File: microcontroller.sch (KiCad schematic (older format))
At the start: 25 parts, among them Q1 DMN62D0U-7, U5 MCP2221A, U6 ESP32, U7 NPIC6C596ADJ, U8 NPIC6C596ADJ, U9 NPIC6C596ADJ

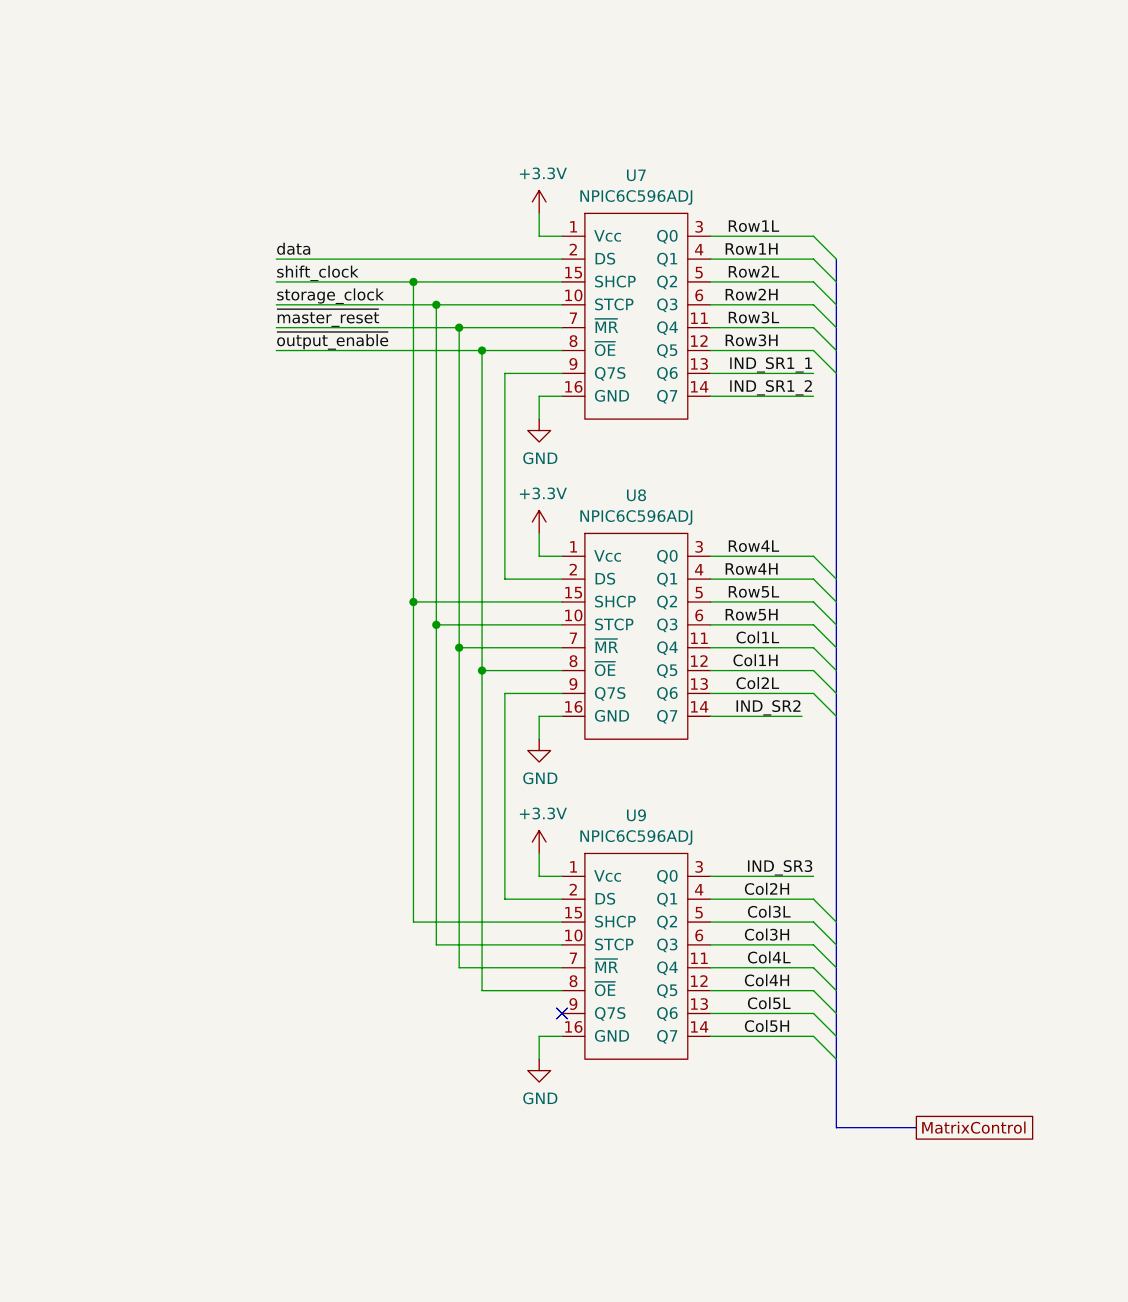
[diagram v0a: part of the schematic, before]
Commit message: more layout work
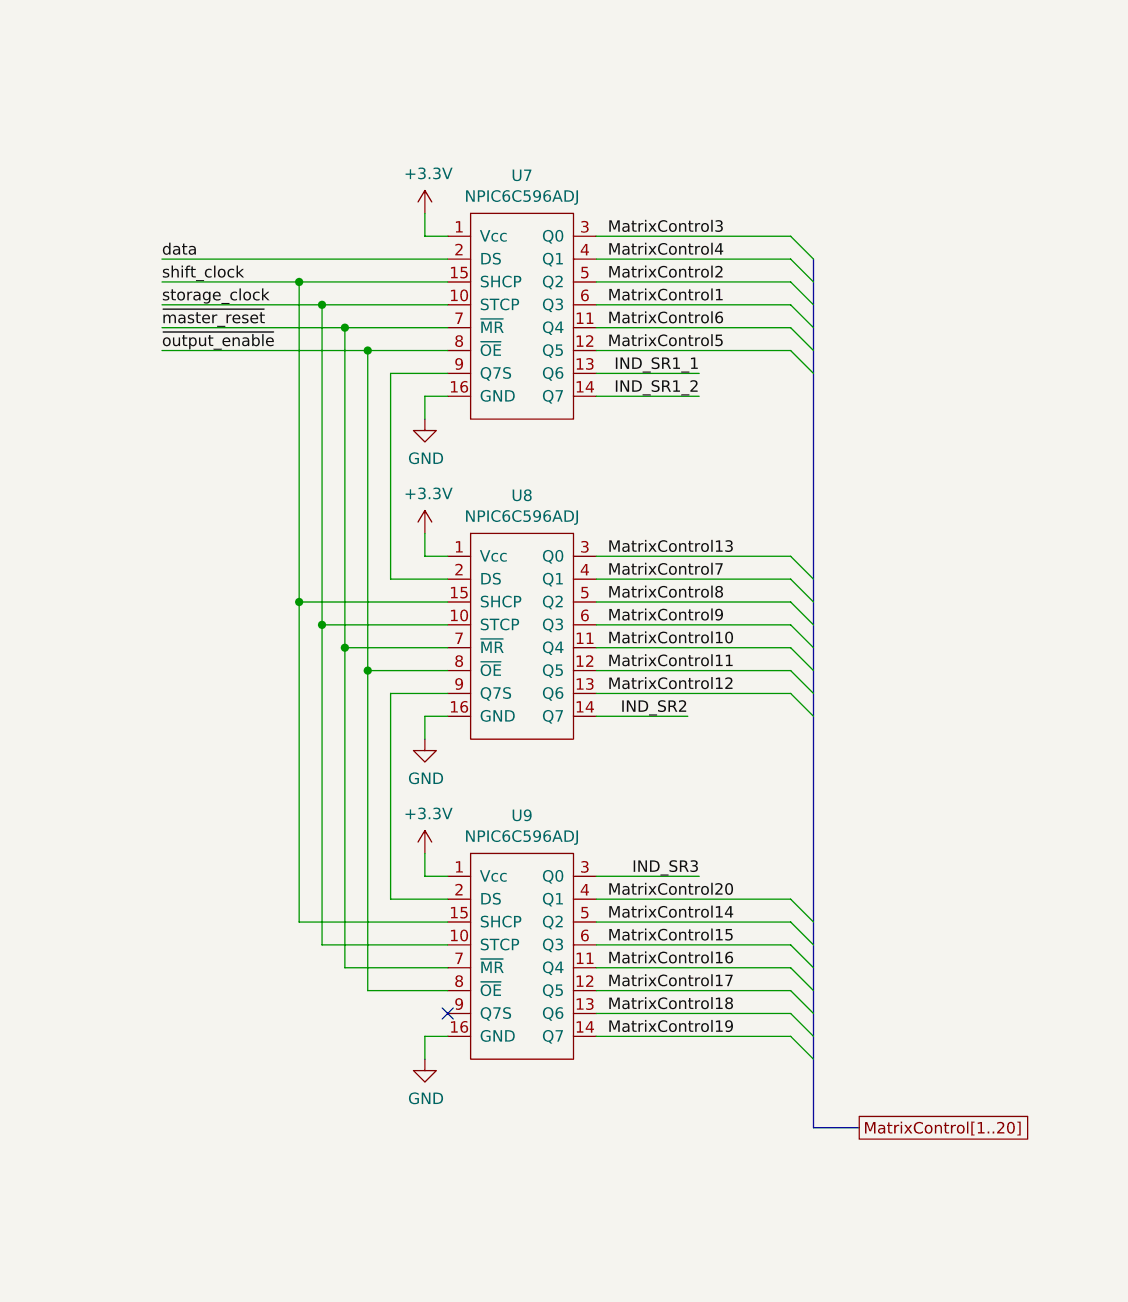
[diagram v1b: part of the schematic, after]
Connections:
- net Col1H renamed MatrixControl11
- net Col1L renamed MatrixControl10
- net Col2H renamed MatrixControl20
- net Col2L renamed MatrixControl12
- net Col3H renamed MatrixControl15
- net Col3L renamed MatrixControl14
- net Col4H renamed MatrixControl17
- net Col4L renamed MatrixControl16
- net Col5H renamed MatrixControl19
- net Col5L renamed MatrixControl18
- net Row1H renamed MatrixControl4
- net Row1L renamed MatrixControl3
- net Row2H renamed MatrixControl1
- net Row2L renamed MatrixControl2
- net Row3H renamed MatrixControl5
- net Row3L renamed MatrixControl6
- net Row4H renamed MatrixControl7
- net Row4L renamed MatrixControl13
- net Row5H renamed MatrixControl9
- net Row5L renamed MatrixControl8
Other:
- moved on the sheet: U7, U8, U9
